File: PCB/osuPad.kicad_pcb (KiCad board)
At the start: 2 copper layers, 85 x 50 mm, 8 parts, among them J1 OLED_128x32, U1 MCU_Seeed_XIAO_RP2040

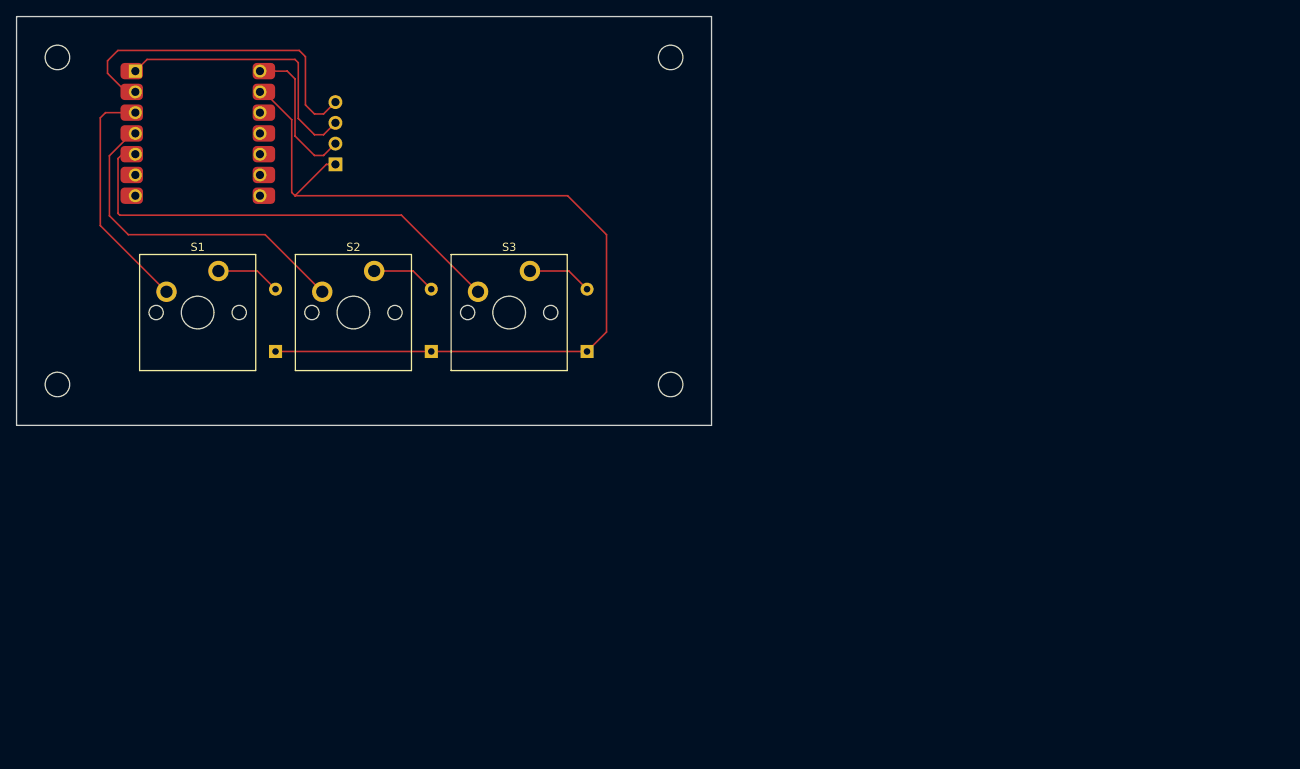
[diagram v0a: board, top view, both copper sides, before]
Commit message: update pcb, case, and readme
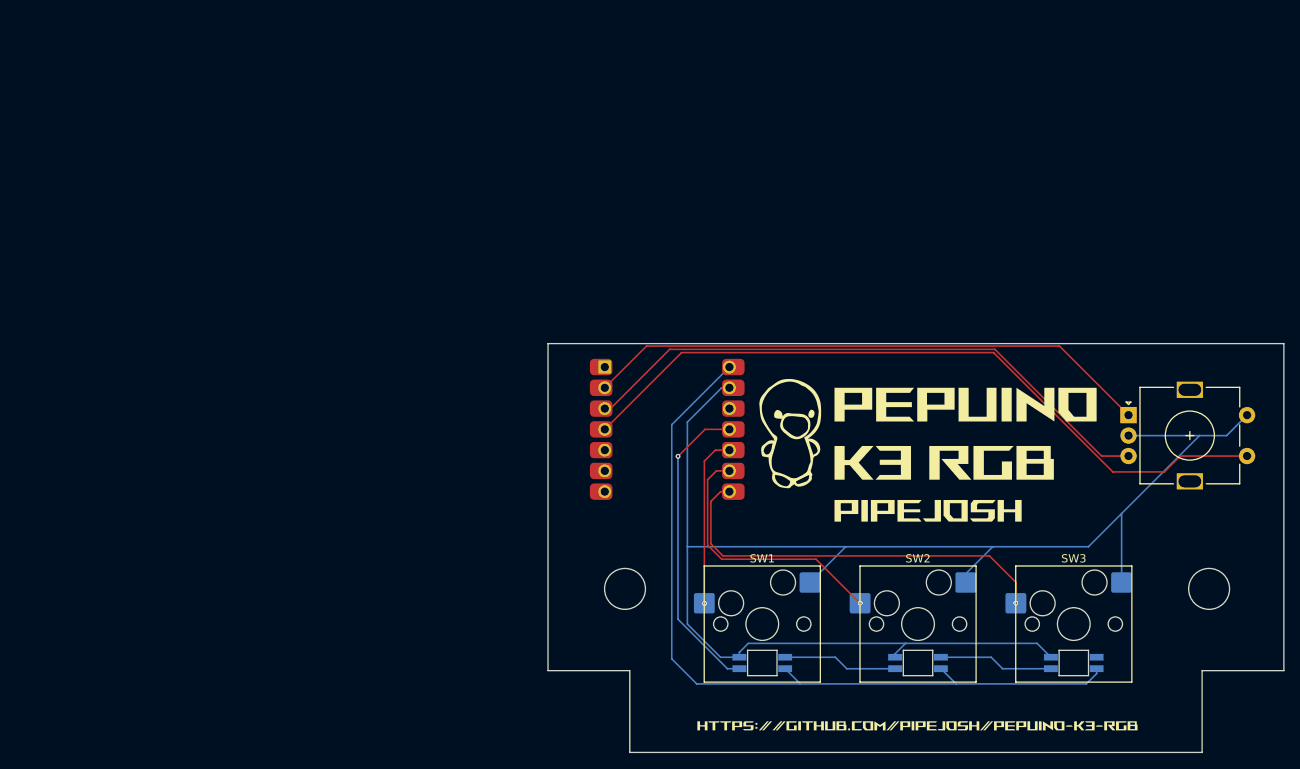
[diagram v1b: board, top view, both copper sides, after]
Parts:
- removed D1, D2, D3: ~, ScottoKeebs_Components:Diode_DO-35
- removed J1: OLED_128x32, ScottoKeebs_Components:OLED_128x32
- removed S1, S2, S3: ~, ScottoKeebs_MX:MX_PCB_1.00u
- added LED1: YS-SK6812MINI-E, kbd:YS-SK6812MINI-E, B.Cu at (126.2, 119.1)
- added LED2: YS-SK6812MINI-E, kbd:YS-SK6812MINI-E, B.Cu at (145.3, 119.1)
- added LED3: YS-SK6812MINI-E, kbd:YS-SK6812MINI-E, B.Cu at (164.3, 119.1)
- added SW1: SW_Push, ScottoKeebs_Hotswap:Hotswap_MX_1.00u, F.Cu at (126.2, 114.3)
- added SW2: SW_Push, ScottoKeebs_Hotswap:Hotswap_MX_1.00u, F.Cu at (145.3, 114.3)
- added SW3: SW_Push, ScottoKeebs_Hotswap:Hotswap_MX_1.00u, F.Cu at (164.3, 114.3)
- added SW4: RotaryEncoder_Switch, Rotary_Encoder:RotaryEncoder_Alps_EC11E-Switch_Vertical_H20mm, F.Cu at (171.0, 88.8)
- moved U1 67.9 mm to (114.6, 90.5)
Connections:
- net Net-(U1-PA9_A5_D5_SCL) renamed SCL
- U1 pad 1: Net-(J1-SCL) -> unconnected-(U1-PA02_A0_D0-Pad1)
- U1 pad 10: unconnected-(U1-PA5_A9_D9_MISO-Pad10) -> SW2
- U1 pad 11: unconnected-(U1-PA6_A10_D10_MOSI-Pad11) -> LED
- U1 pad 12: unconnected-(U1-3V3-Pad12) -> 3V3
- U1 pad 13: Net-(D1-K) -> GND
- U1 pad 14: Net-(J1-VCC) -> VCC
- U1 pad 2: Net-(J1-SDA) -> ENCODER1
- U1 pad 3: Net-(U1-PA10_A2_D2) -> ENCODER2
- U1 pad 4: Net-(U1-PA11_A3_D3) -> ENCODER3
- U1 pad 5: Net-(U1-PA8_A4_D4_SDA) -> SDA
- U1 pad 8: Net-(U1-PB09_A7_D7_RX) -> SW4
- U1 pad 9: Net-(U1-PA7_A8_D8_SCK) -> SW3
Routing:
- net GND: track 0.00 -> 184.8 mm
- net Net-(D1-K): track 114.3 -> 0.00 mm
- net VCC: track 0.00 -> 98.2 mm
- net ENCODER3: track 0.00 -> 89.3 mm
- net ENCODER2: track 0.00 -> 71.8 mm
- net ENCODER1: track 0.00 -> 69.7 mm
- net Net-(U1-PA8_A4_D4_SDA): track 57.1 -> 0.00 mm
- net SW4: track 0.00 -> 49.8 mm, vias 0 -> 1
- net Net-(J1-SDA): track 42.2 -> 0.00 mm
- net Net-(U1-PA11_A3_D3): track 41.1 -> 0.00 mm
- net LED: track 0.00 -> 37.6 mm, vias 0 -> 1
- net Net-(J1-SCL): track 33.5 -> 0.00 mm
- net SW3: track 0.00 -> 32.7 mm, vias 0 -> 1
- net Net-(U1-PA10_A2_D2): track 28.7 -> 0.00 mm
- net SW2: track 0.00 -> 21.0 mm, vias 0 -> 1
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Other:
- board size 85 x 50 mm -> 90 x 50 mm
